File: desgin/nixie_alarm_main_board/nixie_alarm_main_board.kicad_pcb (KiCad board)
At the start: 2 copper layers, 138.3 x 52.9 mm, 116 parts, among them IC1 LM3488MM, IC2 HV5530PG-G, IC3 TPS563219ADDFR, IC4 HV5530PG-G, IC6 CD40109BQNSRQ1, IC7 AP7363-33D-13, IC8 MCP4018T-502E_LT, J1 PJ-094H-SMT-TR, J2 JST XH 2.54 3 pin, J3 USB_C_Receptacle_USB2.0_16P, J5 Goldpin 3pin, Q1 SSM3K35AMFV,L3F, Q2 DMN60H080DS-13, Q3 DMN60H080DS-13, Q4 DMN60H080DS-13, Q5 DMN60H080DS-13, Q6 DMN60H080DS-13, Q7 DMN60H080DS-13, Q8 TPH5200FNH,L1Q, U1 ESP32-S3-WROOM-1

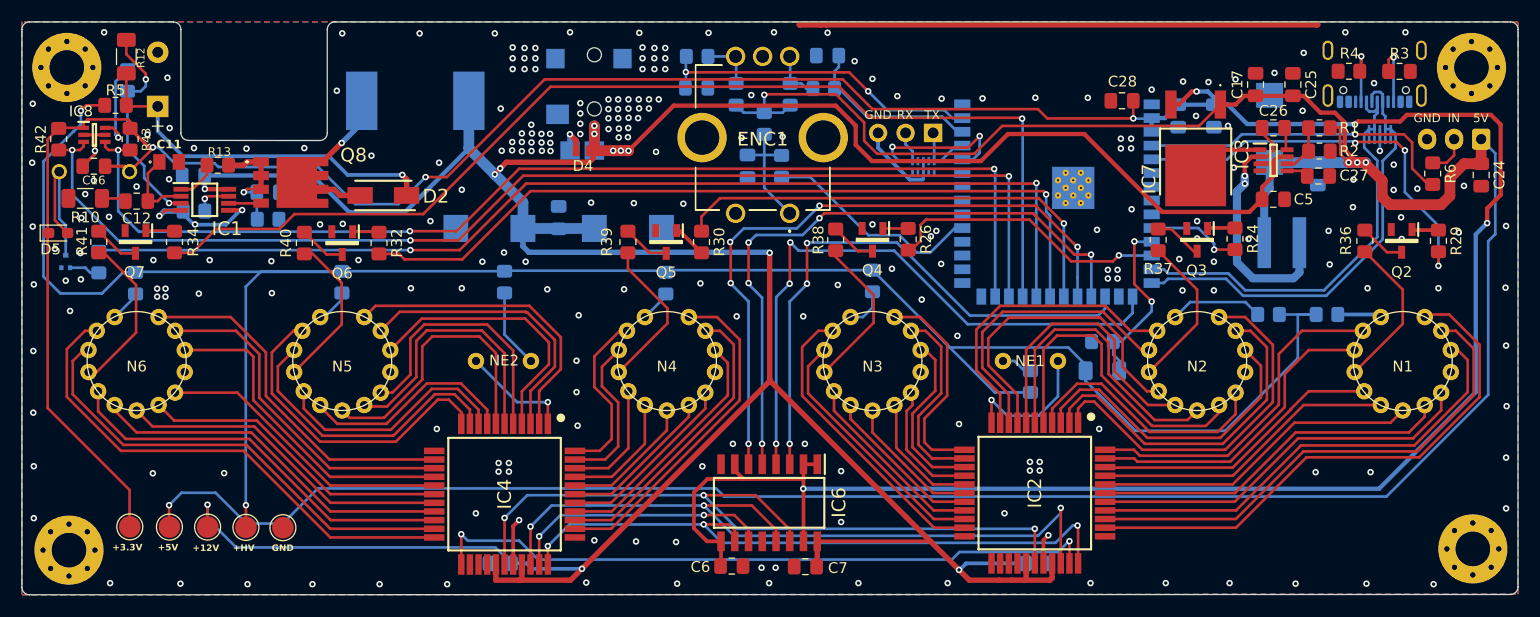
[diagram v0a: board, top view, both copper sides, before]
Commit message: new border
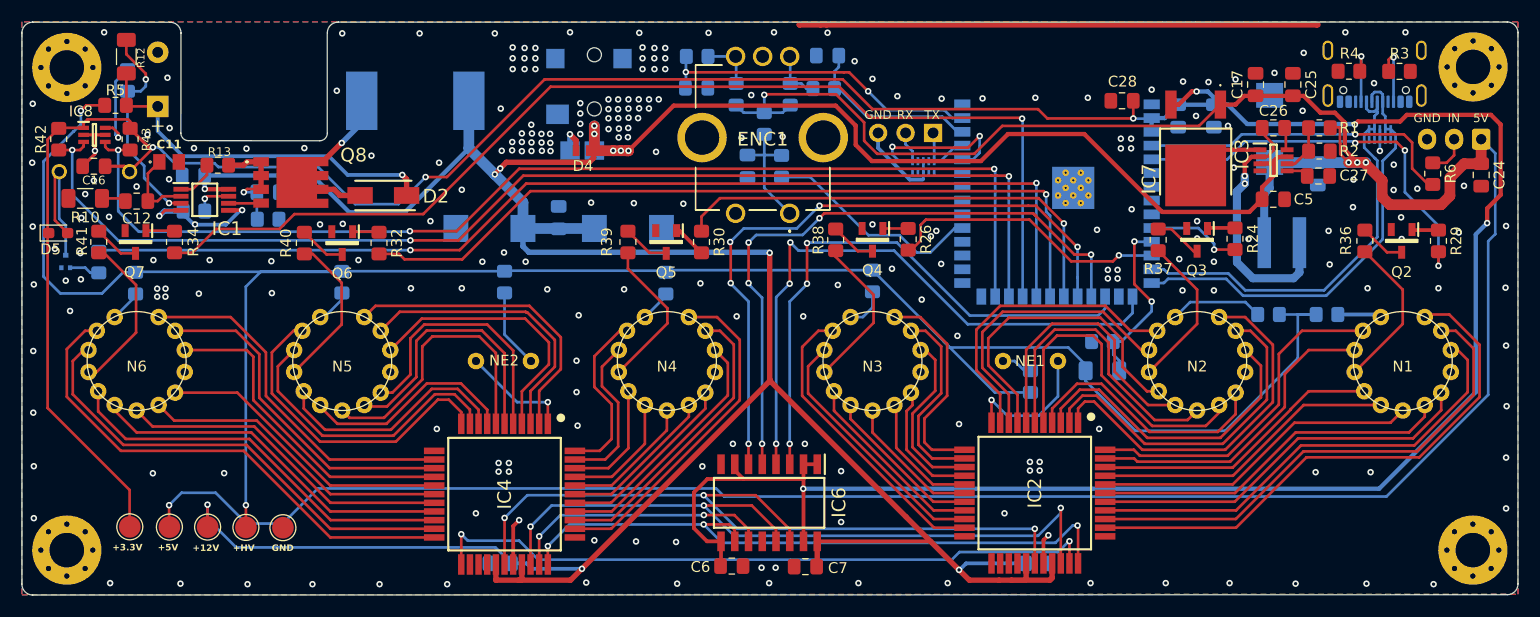
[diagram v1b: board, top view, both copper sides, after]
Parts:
- moved H3 0.20 mm to (91.0, 122.4)
- moved H2 0.16 mm to (220.9, 77.8)
- moved H4 0.11 mm to (220.9, 122.4)
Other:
- outline, holes or cut-outs redrawn
